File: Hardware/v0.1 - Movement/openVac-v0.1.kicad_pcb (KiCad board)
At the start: 2 copper layers, 167 x 100 mm, 14 parts, among them J1 Brush Motor 2 (right), J2 Brush Motor 1 (left), J3 Brush Header, J4 Brush Motor Main, J5 Vacuum, J6 Vacuum Header, Q1 IRF540N, Q2 IRF540N, Q4 IRF540N

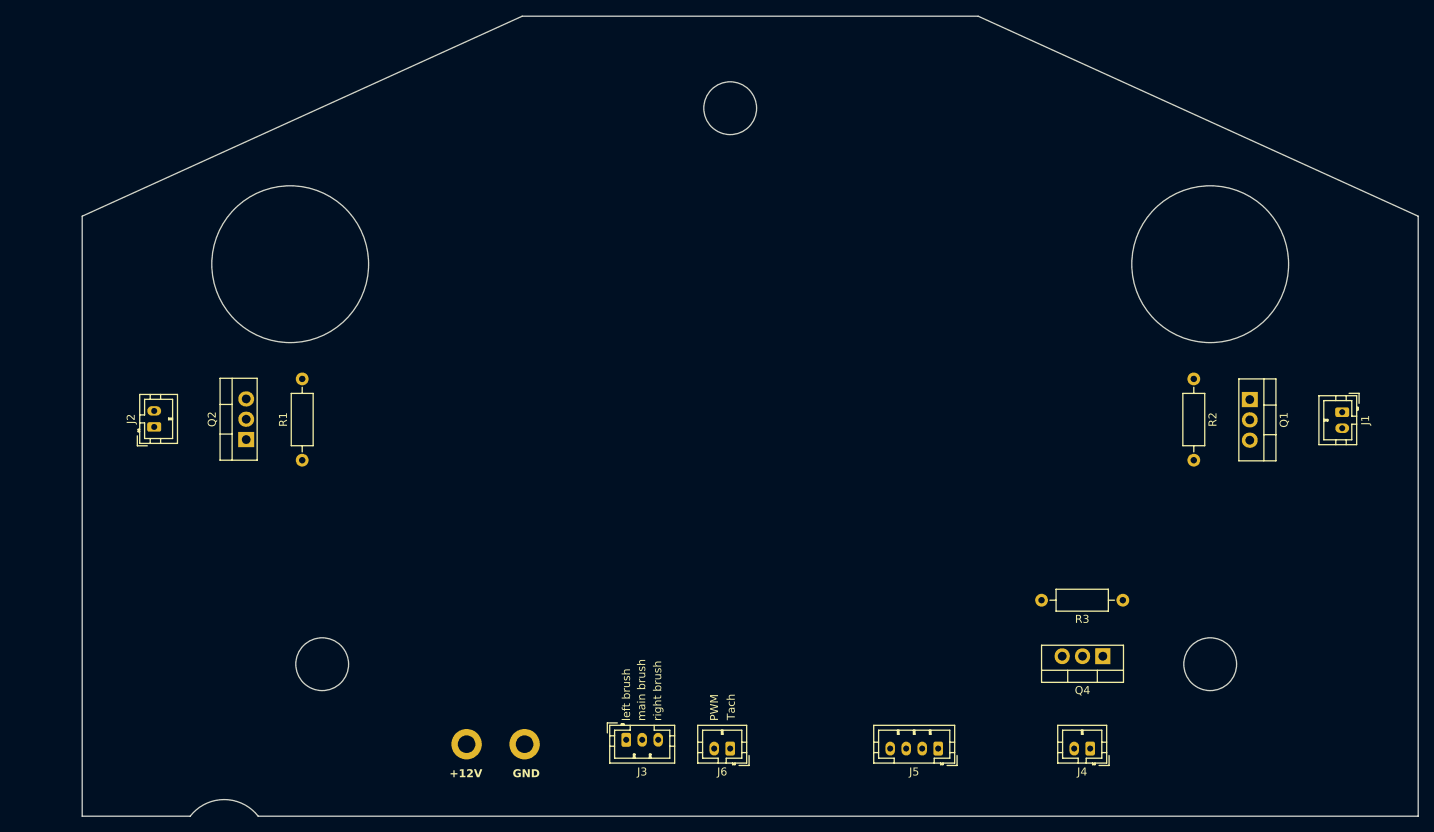
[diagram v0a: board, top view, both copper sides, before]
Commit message: Github Desktop Backup
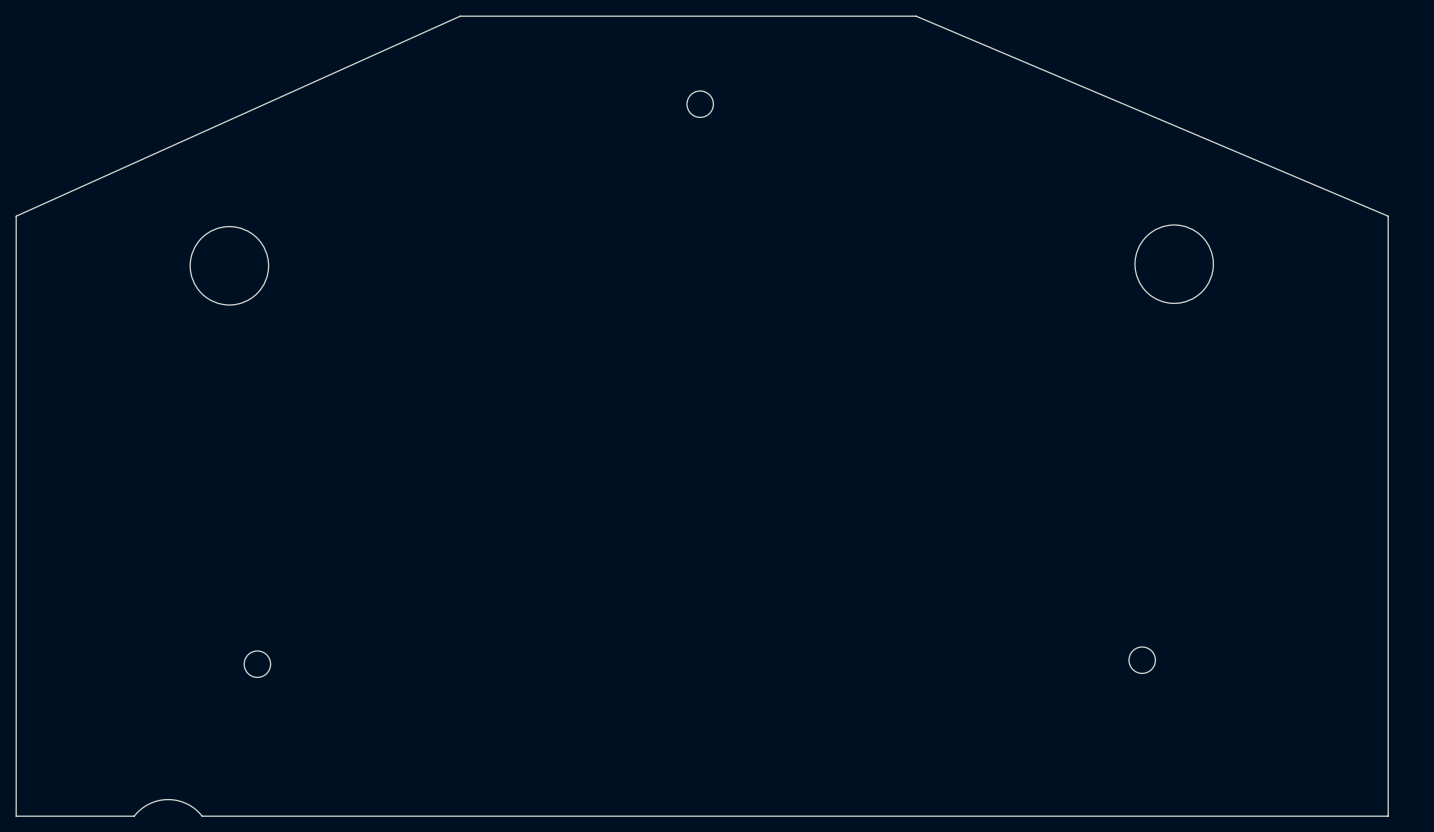
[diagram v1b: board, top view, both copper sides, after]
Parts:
- removed H1: 12V (external in), MountingHole:MountingHole_2.2mm_M2_DIN965_Pad
- removed H2: GND (external in), MountingHole:MountingHole_2.2mm_M2_DIN965_Pad
- removed J1: Brush Motor 2 (right), Connector_JST:JST_PH_B2B-PH-K_1x02_P2.00mm_Vertical
- removed J2: Brush Motor 1 (left), Connector_JST:JST_PH_B2B-PH-K_1x02_P2.00mm_Vertical
- removed J3: Brush Header, Connector_JST:JST_PH_B3B-PH-K_1x03_P2.00mm_Vertical
- removed J4: Brush Motor Main, Connector_JST:JST_PH_B2B-PH-K_1x02_P2.00mm_Vertical
- removed J5: Vacuum, Connector_JST:JST_PH_B4B-PH-K_1x04_P2.00mm_Vertical
- removed J6: Vacuum Header, Connector_JST:JST_PH_B2B-PH-K_1x02_P2.00mm_Vertical
- removed Q1, Q2, Q4: IRF540N, Package_TO_SOT_THT:TO-220-3_Vertical
- removed R1, R2, R3: 10k, Resistor_THT:R_Axial_DIN0207_L6.3mm_D2.5mm_P10.16mm_Horizontal
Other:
- board size 167 x 100 mm -> 171.5 x 100 mm
- board text removed: "+12V"
- board text removed: "GND"
- board text removed: "PWM"
- board text removed: "Tach"
- board text removed: "left brush"
- board text removed: "main brush"
- board text removed: "right brush"
